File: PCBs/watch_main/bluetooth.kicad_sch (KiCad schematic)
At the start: 23 parts, among them U301 NRF5340-QKAA-R7

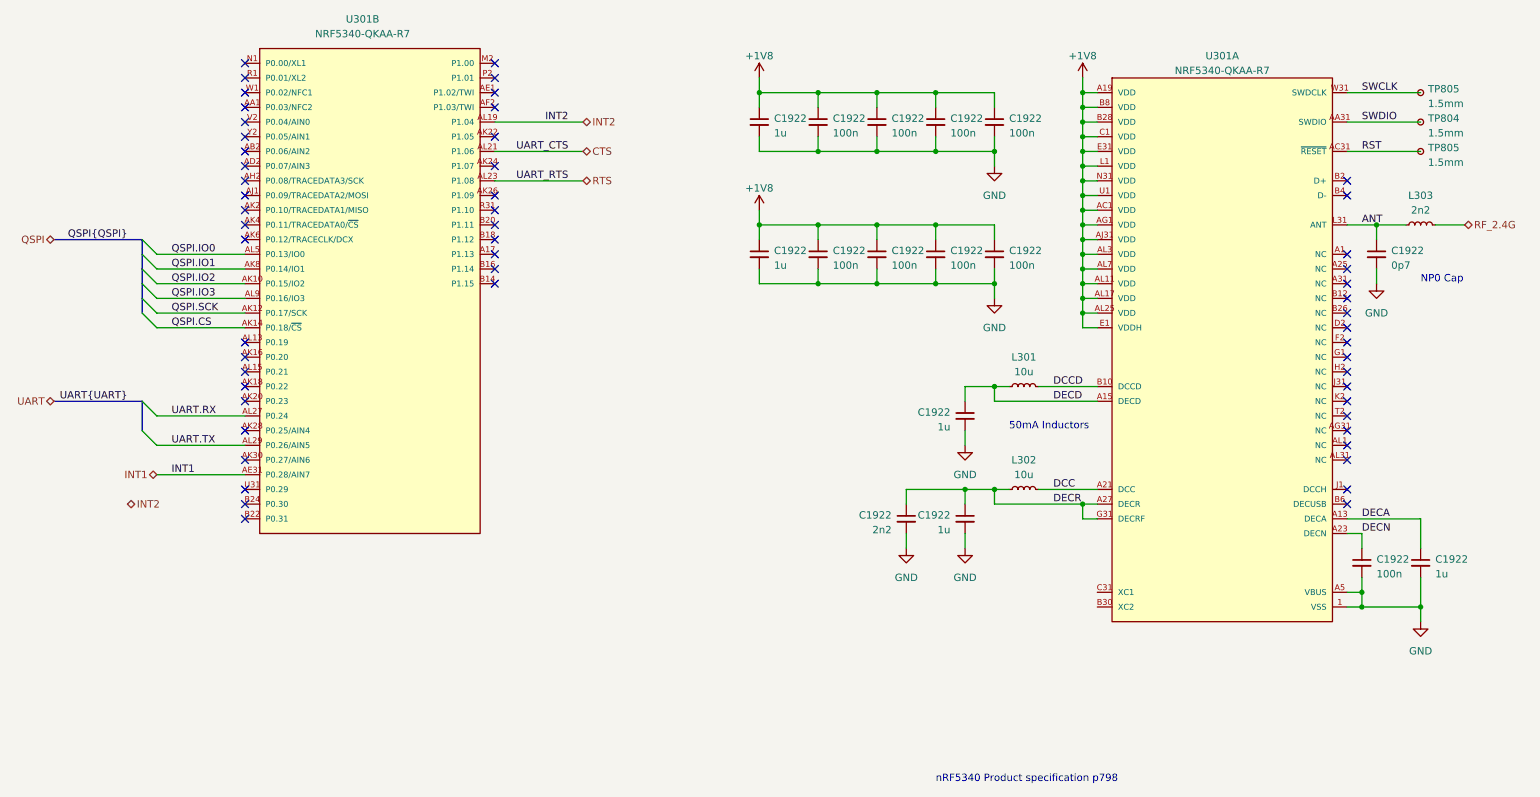
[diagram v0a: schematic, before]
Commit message: PCB Schematic progress
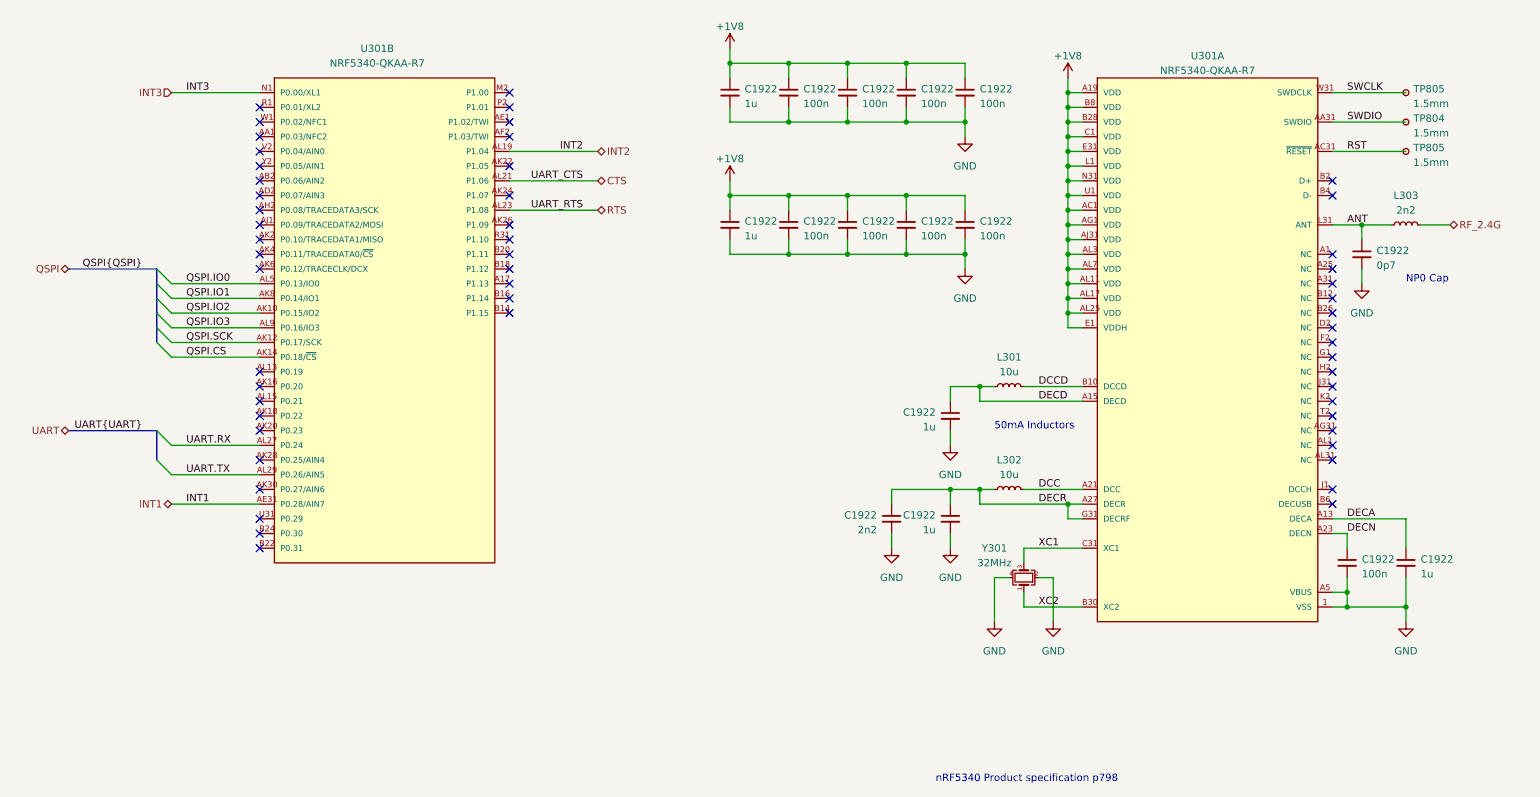
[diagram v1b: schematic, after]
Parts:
- added Y301: 32MHz, Crystal:Crystal_SMD_2016-4Pin_2.0x1.6mm, symbol Device:Crystal_GND24_Small
- U301: footprint watch_footprints:NRF5340-QKAA-R7 -> watch_footprints:NRF5340-QKAA-R7_modified
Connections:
- net GND: now also Y301.2, Y301.4
- net XC2: now reaches U301.B30 (XC2)
- net XC2: now also Y301.1
- net XC1: now reaches U301.C31 (XC1)
- net XC1: now also Y301.3
- net INT3: now reaches U301.N1 (P0.00/XL1)
- no-connect marks 55 -> 54
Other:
- moved on the sheet: C1922, L301, L302, L303, TP804, TP805, U301A, U301B
